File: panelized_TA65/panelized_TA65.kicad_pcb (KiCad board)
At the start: 2 copper layers, 35.6 x 95.6 mm, 172 parts, among them J1 Conn_01x07_Pin, J2 Conn_01x07_Pin

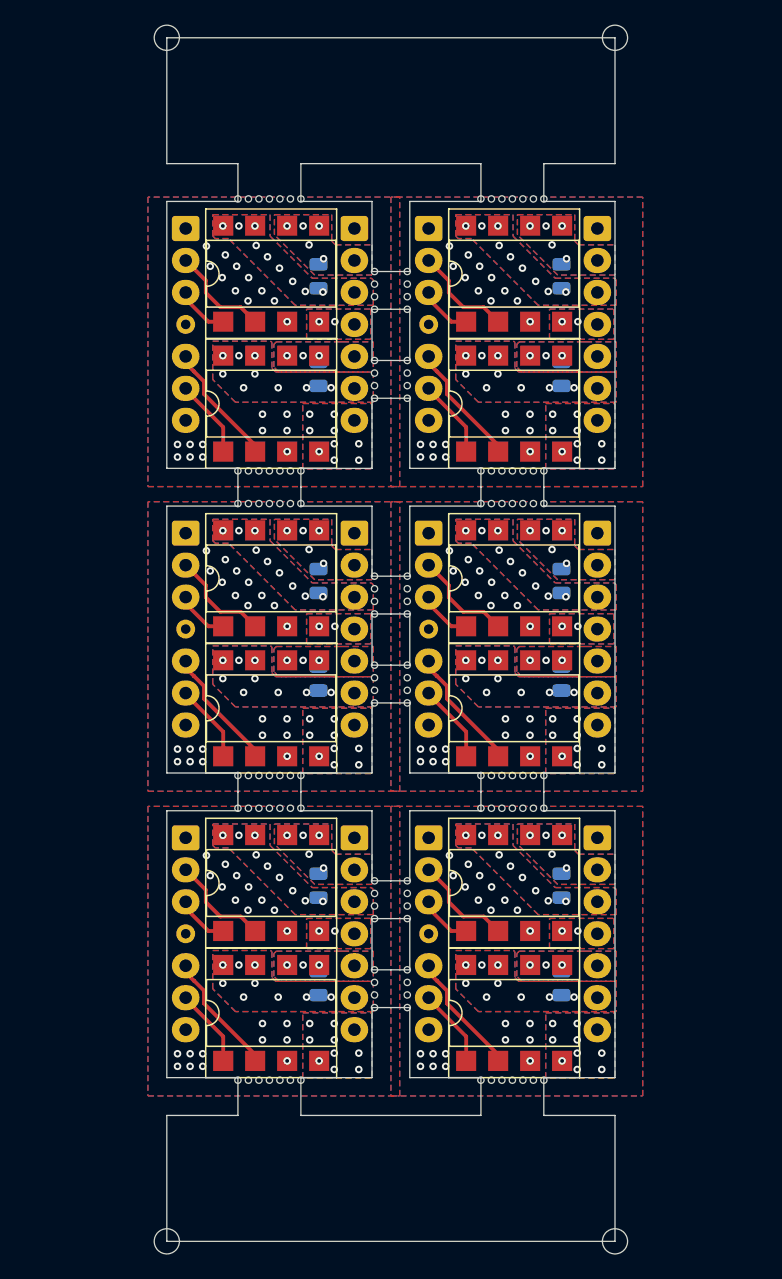
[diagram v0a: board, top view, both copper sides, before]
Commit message: panels
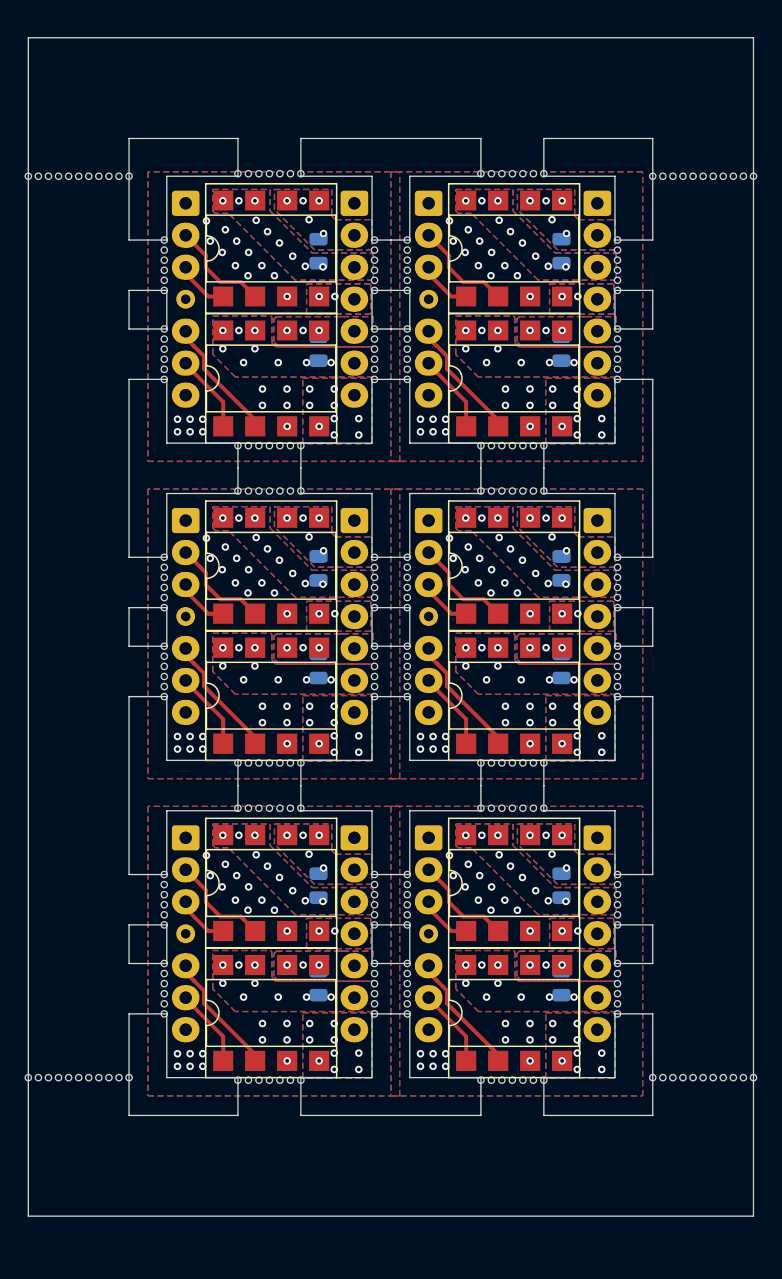
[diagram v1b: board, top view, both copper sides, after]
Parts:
- removed the C1 at (162.1, 63.2)
- removed the C1 at (142.8, 39.0)
- removed the C1 at (142.8, 87.4)
- removed the C1 at (162.1, 39.0)
- removed the C1 at (142.8, 63.2)
- removed the C1 at (162.1, 87.4)
- removed the C2 at (142.8, 46.7)
- removed the C2 at (162.1, 70.9)
- removed the C2 at (162.1, 95.1)
- removed the C2 at (162.1, 46.7)
- removed the C2 at (142.8, 95.1)
- removed the C2 at (142.8, 70.9)
- removed the J1 at (132.2, 35.2)
- removed the J1 at (132.2, 59.4)
- removed the J1 at (132.2, 83.6)
- removed the J1 at (151.5, 59.4)
- removed the J1 at (151.5, 35.2)
- removed the J1 at (151.5, 83.6)
- removed the J2 at (164.9, 83.6)
- removed the J2 at (164.9, 59.4)
- removed the J2 at (164.9, 35.2)
- removed the J2 at (145.6, 83.6)
- removed the J2 at (145.6, 59.4)
- removed the J2 at (145.6, 35.2)
- removed KiKit_MB_15_7, KiKit_MB_16_7, KiKit_MB_19_7, KiKit_MB_20_7, KiKit_MB_3_7, KiKit_MB_4_7, KiKit_MB_7_7, KiKit_MB_8_7, KiKit_TO_1, KiKit_TO_2, KiKit_TO_3, KiKit_TO_4: NPTH, NPTH
- removed the U1 at (158.3, 97.5)
- removed the U1 at (158.3, 49.1)
- removed the U1 at (139.0, 49.1)
- removed the U1 at (139.0, 97.5)
- removed the U1 at (158.3, 73.3)
- removed the U1 at (139.0, 73.3)
- removed the U2 at (158.3, 62.9)
- removed the U2 at (158.3, 38.7)
- removed the U2 at (139.0, 87.1)
- removed the U2 at (139.0, 62.9)
- removed the U2 at (139.0, 38.7)
- removed the U2 at (158.3, 87.1)
- added C1: 100, Capacitor_SMD:C_0805_2012Metric, B.Cu at (142.8, 87.3)
- added C1: 100, Capacitor_SMD:C_0805_2012Metric, B.Cu at (142.8, 62.1)
- added C1: 100, Capacitor_SMD:C_0805_2012Metric, B.Cu at (162.1, 37.0)
- added C1: 100, Capacitor_SMD:C_0805_2012Metric, B.Cu at (142.8, 37.0)
- added C1: 100, Capacitor_SMD:C_0805_2012Metric, B.Cu at (162.1, 87.3)
- added C1: 100, Capacitor_SMD:C_0805_2012Metric, B.Cu at (162.1, 62.1)
- added C2: 100, Capacitor_SMD:C_0805_2012Metric, B.Cu at (162.1, 95.1)
- added C2: 100, Capacitor_SMD:C_0805_2012Metric, B.Cu at (162.1, 44.7)
- added C2: 100, Capacitor_SMD:C_0805_2012Metric, B.Cu at (142.8, 44.7)
- added C2: 100, Capacitor_SMD:C_0805_2012Metric, B.Cu at (142.8, 69.9)
- added C2: 100, Capacitor_SMD:C_0805_2012Metric, B.Cu at (162.1, 69.9)
- added C2: 100, Capacitor_SMD:C_0805_2012Metric, B.Cu at (142.8, 95.1)
- added J1: Conn_01x07_Pin, Connector_PinHeader_2.54mm:PinHeader_1x07_P2.54mm_Vertical, B.Cu at (132.2, 83.5)
- added J1: Conn_01x07_Pin, Connector_PinHeader_2.54mm:PinHeader_1x07_P2.54mm_Vertical, B.Cu at (151.5, 83.5)
- added J1: Conn_01x07_Pin, Connector_PinHeader_2.54mm:PinHeader_1x07_P2.54mm_Vertical, B.Cu at (132.2, 58.4)
- added J1: Conn_01x07_Pin, Connector_PinHeader_2.54mm:PinHeader_1x07_P2.54mm_Vertical, B.Cu at (151.5, 33.1)
- added J1: Conn_01x07_Pin, Connector_PinHeader_2.54mm:PinHeader_1x07_P2.54mm_Vertical, B.Cu at (151.5, 58.4)
- added J1: Conn_01x07_Pin, Connector_PinHeader_2.54mm:PinHeader_1x07_P2.54mm_Vertical, B.Cu at (132.2, 33.1)
- added J2: Conn_01x07_Pin, Connector_PinHeader_2.54mm:PinHeader_1x07_P2.54mm_Vertical, B.Cu at (145.6, 33.1)
- added J2: Conn_01x07_Pin, Connector_PinHeader_2.54mm:PinHeader_1x07_P2.54mm_Vertical, B.Cu at (164.9, 83.5)
- added J2: Conn_01x07_Pin, Connector_PinHeader_2.54mm:PinHeader_1x07_P2.54mm_Vertical, B.Cu at (164.9, 33.1)
- added J2: Conn_01x07_Pin, Connector_PinHeader_2.54mm:PinHeader_1x07_P2.54mm_Vertical, B.Cu at (145.6, 83.5)
- added J2: Conn_01x07_Pin, Connector_PinHeader_2.54mm:PinHeader_1x07_P2.54mm_Vertical, B.Cu at (145.6, 58.4)
- added J2: Conn_01x07_Pin, Connector_PinHeader_2.54mm:PinHeader_1x07_P2.54mm_Vertical, B.Cu at (164.9, 58.4)
- added KiKit_MB_10_5: NPTH, NPTH, F.Cu at (166.5, 46.3)
- added KiKit_MB_10_6: NPTH, NPTH, F.Cu at (166.5, 47.1)
- added KiKit_MB_13_5: NPTH, NPTH, F.Cu at (130.5, 62.1)
- added KiKit_MB_13_6: NPTH, NPTH, F.Cu at (130.5, 61.3)
- added KiKit_MB_14_5: NPTH, NPTH, F.Cu at (130.5, 69.1)
- added KiKit_MB_14_6: NPTH, NPTH, F.Cu at (130.5, 68.3)
- added KiKit_MB_17_5: NPTH, NPTH, F.Cu at (139.7, 56.0)
- added KiKit_MB_17_6: NPTH, NPTH, F.Cu at (140.5, 56.0)
- added KiKit_MB_17_7: NPTH, NPTH, F.Cu at (141.3, 56.0)
- added KiKit_MB_18_5: NPTH, NPTH, F.Cu at (138.0, 77.6)
- added KiKit_MB_18_6: NPTH, NPTH, F.Cu at (137.2, 77.6)
- added KiKit_MB_18_7: NPTH, NPTH, F.Cu at (136.3, 77.6)
- added KiKit_MB_1_5: NPTH, NPTH, F.Cu at (130.5, 36.9)
- added KiKit_MB_1_6: NPTH, NPTH, F.Cu at (130.5, 36.1)
- added KiKit_MB_21_5: NPTH, NPTH, F.Cu at (166.5, 64.5)
- added KiKit_MB_21_6: NPTH, NPTH, F.Cu at (166.5, 65.3)
- added KiKit_MB_22_5: NPTH, NPTH, F.Cu at (166.5, 71.5)
- added KiKit_MB_22_6: NPTH, NPTH, F.Cu at (166.5, 72.3)
- added KiKit_MB_25_1: NPTH, NPTH, F.Cu at (130.5, 90.5)
- added KiKit_MB_25_2: NPTH, NPTH, F.Cu at (130.5, 89.7)
- added KiKit_MB_25_3: NPTH, NPTH, F.Cu at (130.5, 88.9)
- added KiKit_MB_25_4: NPTH, NPTH, F.Cu at (130.5, 88.1)
- added KiKit_MB_25_5: NPTH, NPTH, F.Cu at (130.5, 87.3)
- added KiKit_MB_25_6: NPTH, NPTH, F.Cu at (130.5, 86.5)
- added KiKit_MB_26_1: NPTH, NPTH, F.Cu at (130.5, 97.5)
- added KiKit_MB_26_2: NPTH, NPTH, F.Cu at (130.5, 96.7)
- added KiKit_MB_26_3: NPTH, NPTH, F.Cu at (130.5, 95.9)
- added KiKit_MB_26_4: NPTH, NPTH, F.Cu at (130.5, 95.1)
- added KiKit_MB_26_5: NPTH, NPTH, F.Cu at (130.5, 94.3)
- added KiKit_MB_26_6: NPTH, NPTH, F.Cu at (130.5, 93.5)
- added KiKit_MB_27_1: NPTH, NPTH, F.Cu at (147.2, 86.5)
- added KiKit_MB_27_2: NPTH, NPTH, F.Cu at (147.2, 87.3)
- added KiKit_MB_27_3: NPTH, NPTH, F.Cu at (147.2, 88.1)
- added KiKit_MB_27_4: NPTH, NPTH, F.Cu at (147.2, 88.9)
- added KiKit_MB_27_5: NPTH, NPTH, F.Cu at (147.2, 89.7)
- added KiKit_MB_27_6: NPTH, NPTH, F.Cu at (147.2, 90.5)
- added KiKit_MB_28_1: NPTH, NPTH, F.Cu at (147.2, 93.5)
- added KiKit_MB_28_2: NPTH, NPTH, F.Cu at (147.2, 94.3)
- added KiKit_MB_28_3: NPTH, NPTH, F.Cu at (147.2, 95.1)
- added KiKit_MB_28_4: NPTH, NPTH, F.Cu at (147.2, 95.9)
- added KiKit_MB_28_5: NPTH, NPTH, F.Cu at (147.2, 96.7)
- added KiKit_MB_28_6: NPTH, NPTH, F.Cu at (147.2, 97.5)
- added KiKit_MB_29_1: NPTH, NPTH, F.Cu at (136.3, 81.2)
- added KiKit_MB_29_2: NPTH, NPTH, F.Cu at (137.2, 81.2)
- added KiKit_MB_29_3: NPTH, NPTH, F.Cu at (138.0, 81.2)
- added KiKit_MB_29_4: NPTH, NPTH, F.Cu at (138.8, 81.2)
- added KiKit_MB_29_5: NPTH, NPTH, F.Cu at (139.7, 81.2)
- added KiKit_MB_29_6: NPTH, NPTH, F.Cu at (140.5, 81.2)
- added KiKit_MB_29_7: NPTH, NPTH, F.Cu at (141.3, 81.2)
- added KiKit_MB_2_5: NPTH, NPTH, F.Cu at (130.5, 43.9)
- added KiKit_MB_2_6: NPTH, NPTH, F.Cu at (130.5, 43.1)
- added KiKit_MB_30_1: NPTH, NPTH, F.Cu at (141.3, 102.8)
- added KiKit_MB_30_2: NPTH, NPTH, F.Cu at (140.5, 102.8)
- added KiKit_MB_30_3: NPTH, NPTH, F.Cu at (139.7, 102.8)
- added KiKit_MB_30_4: NPTH, NPTH, F.Cu at (138.8, 102.8)
- added KiKit_MB_30_5: NPTH, NPTH, F.Cu at (138.0, 102.8)
- added KiKit_MB_30_6: NPTH, NPTH, F.Cu at (137.2, 102.8)
- added KiKit_MB_30_7: NPTH, NPTH, F.Cu at (136.3, 102.8)
- added KiKit_MB_31_1: NPTH, NPTH, F.Cu at (149.8, 90.5)
- added KiKit_MB_31_2: NPTH, NPTH, F.Cu at (149.8, 89.7)
- added KiKit_MB_31_3: NPTH, NPTH, F.Cu at (149.8, 88.9)
- added KiKit_MB_31_4: NPTH, NPTH, F.Cu at (149.8, 88.1)
- added KiKit_MB_31_5: NPTH, NPTH, F.Cu at (149.8, 87.3)
- added KiKit_MB_31_6: NPTH, NPTH, F.Cu at (149.8, 86.5)
- added KiKit_MB_32_1: NPTH, NPTH, F.Cu at (149.8, 97.5)
- added KiKit_MB_32_2: NPTH, NPTH, F.Cu at (149.8, 96.7)
- added KiKit_MB_32_3: NPTH, NPTH, F.Cu at (149.8, 95.9)
- added KiKit_MB_32_4: NPTH, NPTH, F.Cu at (149.8, 95.1)
- added KiKit_MB_32_5: NPTH, NPTH, F.Cu at (149.8, 94.3)
- added KiKit_MB_32_6: NPTH, NPTH, F.Cu at (149.8, 93.5)
- added KiKit_MB_33_1: NPTH, NPTH, F.Cu at (166.5, 86.5)
- added KiKit_MB_33_2: NPTH, NPTH, F.Cu at (166.5, 87.3)
- added KiKit_MB_33_3: NPTH, NPTH, F.Cu at (166.5, 88.1)
- added KiKit_MB_33_4: NPTH, NPTH, F.Cu at (166.5, 88.9)
- added KiKit_MB_33_5: NPTH, NPTH, F.Cu at (166.5, 89.7)
- added KiKit_MB_33_6: NPTH, NPTH, F.Cu at (166.5, 90.5)
- added KiKit_MB_34_1: NPTH, NPTH, F.Cu at (166.5, 93.5)
- added KiKit_MB_34_2: NPTH, NPTH, F.Cu at (166.5, 94.3)
- added KiKit_MB_34_3: NPTH, NPTH, F.Cu at (166.5, 95.1)
- added KiKit_MB_34_4: NPTH, NPTH, F.Cu at (166.5, 95.9)
- added KiKit_MB_34_5: NPTH, NPTH, F.Cu at (166.5, 96.7)
- added KiKit_MB_34_6: NPTH, NPTH, F.Cu at (166.5, 97.5)
- added KiKit_MB_35_1: NPTH, NPTH, F.Cu at (155.7, 81.2)
- added KiKit_MB_35_2: NPTH, NPTH, F.Cu at (156.5, 81.2)
- added KiKit_MB_35_3: NPTH, NPTH, F.Cu at (157.3, 81.2)
- added KiKit_MB_35_4: NPTH, NPTH, F.Cu at (158.2, 81.2)
- added KiKit_MB_35_5: NPTH, NPTH, F.Cu at (159.0, 81.2)
- added KiKit_MB_35_6: NPTH, NPTH, F.Cu at (159.8, 81.2)
- added KiKit_MB_35_7: NPTH, NPTH, F.Cu at (160.7, 81.2)
- added KiKit_MB_36_1: NPTH, NPTH, F.Cu at (160.7, 102.8)
- added KiKit_MB_36_2: NPTH, NPTH, F.Cu at (159.8, 102.8)
- added KiKit_MB_36_3: NPTH, NPTH, F.Cu at (159.0, 102.8)
- added KiKit_MB_36_4: NPTH, NPTH, F.Cu at (158.2, 102.8)
- added KiKit_MB_36_5: NPTH, NPTH, F.Cu at (157.3, 102.8)
- added KiKit_MB_36_6: NPTH, NPTH, F.Cu at (156.5, 102.8)
- added KiKit_MB_36_7: NPTH, NPTH, F.Cu at (155.7, 102.8)
- added KiKit_MB_37_1: NPTH, NPTH, F.Cu at (119.7, 31.0)
- added KiKit_MB_37_10: NPTH, NPTH, F.Cu at (126.9, 31.0)
- added KiKit_MB_37_11: NPTH, NPTH, F.Cu at (127.7, 31.0)
- added KiKit_MB_37_2: NPTH, NPTH, F.Cu at (120.5, 31.0)
- added KiKit_MB_37_3: NPTH, NPTH, F.Cu at (121.3, 31.0)
- added KiKit_MB_37_4: NPTH, NPTH, F.Cu at (122.1, 31.0)
- added KiKit_MB_37_5: NPTH, NPTH, F.Cu at (122.9, 31.0)
- added KiKit_MB_37_6: NPTH, NPTH, F.Cu at (123.7, 31.0)
- added KiKit_MB_37_7: NPTH, NPTH, F.Cu at (124.5, 31.0)
- added KiKit_MB_37_8: NPTH, NPTH, F.Cu at (125.3, 31.0)
- added KiKit_MB_37_9: NPTH, NPTH, F.Cu at (126.1, 31.0)
- added KiKit_MB_38_1: NPTH, NPTH, F.Cu at (119.7, 102.6)
- added KiKit_MB_38_10: NPTH, NPTH, F.Cu at (126.9, 102.6)
- added KiKit_MB_38_11: NPTH, NPTH, F.Cu at (127.7, 102.6)
- added KiKit_MB_38_2: NPTH, NPTH, F.Cu at (120.5, 102.6)
- added KiKit_MB_38_3: NPTH, NPTH, F.Cu at (121.3, 102.6)
- added KiKit_MB_38_4: NPTH, NPTH, F.Cu at (122.1, 102.6)
- added KiKit_MB_38_5: NPTH, NPTH, F.Cu at (122.9, 102.6)
- added KiKit_MB_38_6: NPTH, NPTH, F.Cu at (123.7, 102.6)
- added KiKit_MB_38_7: NPTH, NPTH, F.Cu at (124.5, 102.6)
- added KiKit_MB_38_8: NPTH, NPTH, F.Cu at (125.3, 102.6)
- added KiKit_MB_38_9: NPTH, NPTH, F.Cu at (126.1, 102.6)
- added KiKit_MB_39_1: NPTH, NPTH, F.Cu at (169.3, 31.0)
- added KiKit_MB_39_10: NPTH, NPTH, F.Cu at (176.5, 31.0)
- added KiKit_MB_39_11: NPTH, NPTH, F.Cu at (177.3, 31.0)
- added KiKit_MB_39_2: NPTH, NPTH, F.Cu at (170.1, 31.0)
- added KiKit_MB_39_3: NPTH, NPTH, F.Cu at (170.9, 31.0)
- added KiKit_MB_39_4: NPTH, NPTH, F.Cu at (171.7, 31.0)
- added KiKit_MB_39_5: NPTH, NPTH, F.Cu at (172.5, 31.0)
- added KiKit_MB_39_6: NPTH, NPTH, F.Cu at (173.3, 31.0)
- added KiKit_MB_39_7: NPTH, NPTH, F.Cu at (174.1, 31.0)
- added KiKit_MB_39_8: NPTH, NPTH, F.Cu at (174.9, 31.0)
- added KiKit_MB_39_9: NPTH, NPTH, F.Cu at (175.7, 31.0)
- added KiKit_MB_40_1: NPTH, NPTH, F.Cu at (169.3, 102.6)
- added KiKit_MB_40_10: NPTH, NPTH, F.Cu at (176.5, 102.6)
- added KiKit_MB_40_11: NPTH, NPTH, F.Cu at (177.3, 102.6)
- added KiKit_MB_40_2: NPTH, NPTH, F.Cu at (170.1, 102.6)
- added KiKit_MB_40_3: NPTH, NPTH, F.Cu at (170.9, 102.6)
- added KiKit_MB_40_4: NPTH, NPTH, F.Cu at (171.7, 102.6)
- added KiKit_MB_40_5: NPTH, NPTH, F.Cu at (172.5, 102.6)
- added KiKit_MB_40_6: NPTH, NPTH, F.Cu at (173.3, 102.6)
- added KiKit_MB_40_7: NPTH, NPTH, F.Cu at (174.1, 102.6)
- added KiKit_MB_40_8: NPTH, NPTH, F.Cu at (174.9, 102.6)
- added KiKit_MB_40_9: NPTH, NPTH, F.Cu at (175.7, 102.6)
- added KiKit_MB_5_5: NPTH, NPTH, F.Cu at (139.7, 30.8)
- added KiKit_MB_5_6: NPTH, NPTH, F.Cu at (140.5, 30.8)
- added KiKit_MB_5_7: NPTH, NPTH, F.Cu at (141.3, 30.8)
- added KiKit_MB_6_5: NPTH, NPTH, F.Cu at (138.0, 52.4)
- added KiKit_MB_6_6: NPTH, NPTH, F.Cu at (137.2, 52.4)
- added KiKit_MB_6_7: NPTH, NPTH, F.Cu at (136.3, 52.4)
- added KiKit_MB_9_5: NPTH, NPTH, F.Cu at (166.5, 39.3)
- added KiKit_MB_9_6: NPTH, NPTH, F.Cu at (166.5, 40.1)
- added U1: ~, Package_DIP:DIP-8_W7.62mm_SMDSocket_SmallPads, F.Cu at (139.0, 97.5)
- added U1: ~, Package_DIP:DIP-8_W7.62mm_SMDSocket_SmallPads, F.Cu at (158.3, 97.5)
- added U1: ~, Package_DIP:DIP-8_W7.62mm_SMDSocket_SmallPads, F.Cu at (158.3, 47.1)
- added U1: ~, Package_DIP:DIP-8_W7.62mm_SMDSocket_SmallPads, F.Cu at (139.0, 47.1)
- added U1: ~, Package_DIP:DIP-8_W7.62mm_SMDSocket_SmallPads, F.Cu at (139.0, 72.3)
- added U1: ~, Package_DIP:DIP-8_W7.62mm_SMDSocket_SmallPads, F.Cu at (158.3, 72.3)
- added U2: ~, Package_DIP:DIP-8_W7.62mm_SMDSocket_SmallPads, F.Cu at (158.3, 36.7)
- added U2: ~, Package_DIP:DIP-8_W7.62mm_SMDSocket_SmallPads, F.Cu at (139.0, 61.9)
- added U2: ~, Package_DIP:DIP-8_W7.62mm_SMDSocket_SmallPads, F.Cu at (139.0, 36.7)
- added U2: ~, Package_DIP:DIP-8_W7.62mm_SMDSocket_SmallPads, F.Cu at (158.3, 87.1)
- added U2: ~, Package_DIP:DIP-8_W7.62mm_SMDSocket_SmallPads, F.Cu at (158.3, 61.9)
- added U2: ~, Package_DIP:DIP-8_W7.62mm_SMDSocket_SmallPads, F.Cu at (139.0, 87.1)
- moved KiKit_MB_20_6 36.7 mm to (149.8, 68.3)
- moved KiKit_MB_20_5 35.7 mm to (149.8, 69.1)
- moved KiKit_MB_17_4 35.0 mm to (138.8, 56.0)
- moved KiKit_MB_20_4 34.6 mm to (149.8, 69.9)
- moved KiKit_MB_17_3 34.2 mm to (138.0, 56.0)
- moved KiKit_MB_20_3 33.6 mm to (149.8, 70.7)
- moved KiKit_MB_17_2 33.5 mm to (137.2, 56.0)
- moved KiKit_MB_10_4 33.4 mm to (166.5, 45.5)
- moved KiKit_MB_9_4 33.4 mm to (166.5, 38.5)
- moved KiKit_MB_10_3 33.3 mm to (166.5, 44.7)
- moved KiKit_MB_9_3 33.3 mm to (166.5, 37.7)
- moved KiKit_MB_21_1 33.2 mm to (166.5, 61.3)
- moved KiKit_MB_22_1 33.2 mm to (166.5, 68.3)
- moved KiKit_MB_10_2 33.1 mm to (166.5, 43.9)
- moved KiKit_MB_9_2 33.1 mm to (166.5, 36.9)
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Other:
- board size 35.6 x 95.6 mm -> 57.6 x 93.6 mm
